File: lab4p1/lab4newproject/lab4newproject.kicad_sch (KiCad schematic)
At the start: 10 parts, among them J1 9V, U1 NE555D

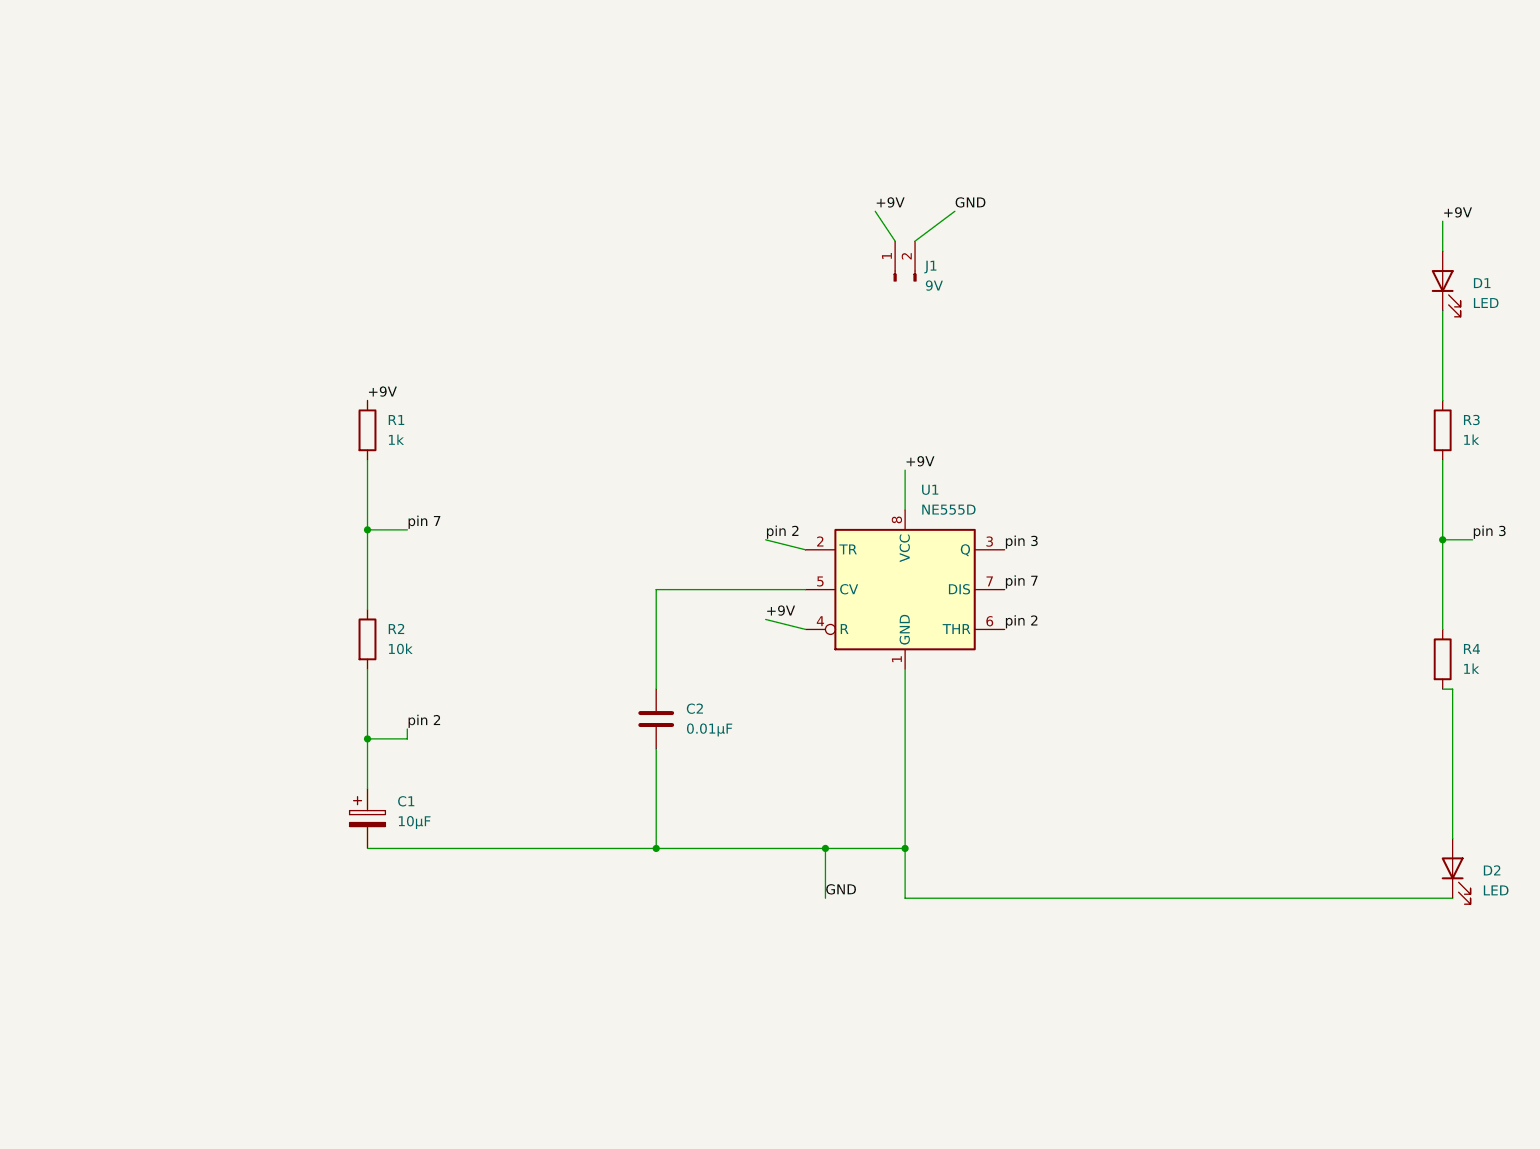
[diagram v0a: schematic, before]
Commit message: PCB design pics
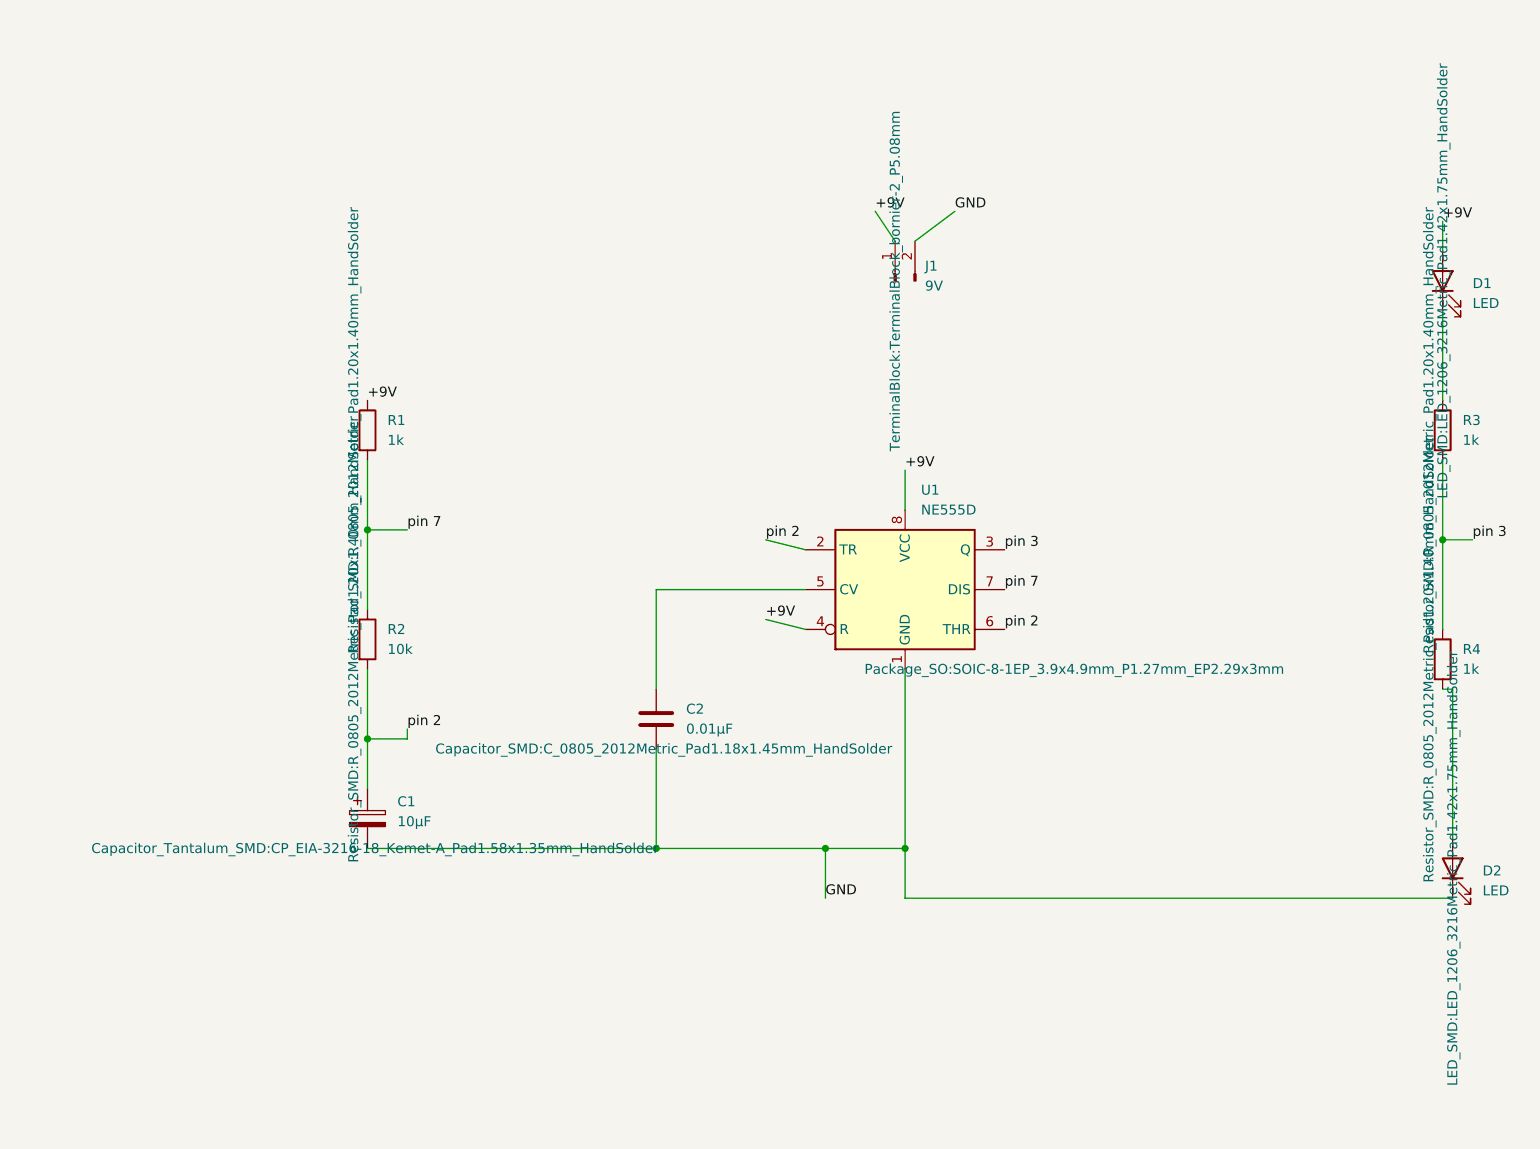
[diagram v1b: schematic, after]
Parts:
- C1: footprint (none) -> Capacitor_Tantalum_SMD:CP_EIA-3216-18_Kemet-A_Pad1.58x1.35mm_HandSolder
- C2: footprint (none) -> Capacitor_SMD:C_0805_2012Metric_Pad1.18x1.45mm_HandSolder
- D1, D2: footprint (none) -> LED_SMD:LED_1206_3216Metric_Pad1.42x1.75mm_HandSolder
- J1: footprint (none) -> TerminalBlock:TerminalBlock_bornier-2_P5.08mm
- R1, R2, R3, R4: footprint (none) -> Resistor_SMD:R_0805_2012Metric_Pad1.20x1.40mm_HandSolder
- U1: footprint Package_SO:SOIC-8_3.9x4.9mm_P1.27mm -> Package_SO:SOIC-8-1EP_3.9x4.9mm_P1.27mm_EP2.29x3mm
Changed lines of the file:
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@@
       (effects (font (size 1.27 1.27)) (justify right))
     )
-    (property "Footprint" "" (id 2) (at 207.01 34.29 0)
-      (effects (font (size 1.27 1.27)) hide)
-    )
+    (property "Footprint" "LED_SMD:LED_1206_3216Metric_Pad1.42x1.75mm_HandSolder" (id 2) (at 207.01 34.29 0))
     (property "Datasheet" "~" (id 3) (at 207.01 34.29 0)
       (effects (font (size 1.27 1.27)) hide)
@@
       (effects (font (size 1.27 1.27)) (justify right))
     )
-    (property "Footprint" "" (id 2) (at 137.16 34.29 0)
-      (effects (font (size 1.27 1.27)) hide)
-    )
+    (property "Footprint" "TerminalBlock:TerminalBlock_bornier-2_P5.08mm" (id 2) (at 137.16 34.29 0))
     (property "Datasheet" "~" (id 3) (at 137.16 34.29 0)
       (effects (font (size 1.27 1.27)) hide)
@@
       (effects (font (size 1.27 1.27)) (justify right))
     )
-    (property "Footprint" "" (id 2) (at 208.28 109.22 0)
-      (effects (font (size 1.27 1.27)) hide)
-    )
+    (property "Footprint" "LED_SMD:LED_1206_3216Metric_Pad1.42x1.75mm_HandSolder" (id 2) (at 208.28 109.22 0))
     (property "Datasheet" "~" (id 3) (at 208.28 109.22 0)
       (effects (font (size 1.27 1.27)) hide)
@@
       (effects (font (size 1.27 1.27)) (justify left))
     )
-    (property "Footprint" "" (id 2) (at 205.232 82.55 90)
-      (effects (font (size 1.27 1.27)) hide)
-    )
+    (property "Footprint" "Resistor_SMD:R_0805_2012Metric_Pad1.20x1.40mm_HandSolder" (id 2) (at 205.232 82.55 90))
     (property "Datasheet" "~" (id 3) (at 207.01 82.55 0)
       (effects (font (size 1.27 1.27)) hide)
@@
       (effects (font (size 1.27 1.27)) (justify left))
     )
-    (property "Footprint" "" (id 2) (at 70.8152 106.68 0)
-      (effects (font (size 1.27 1.27)) hide)
-    )
+    (property "Footprint" "Capacitor_Tantalum_SMD:CP_EIA-3216-18_Kemet-A_Pad1.58x1.35mm_HandSolder" (id 2) (at 70.8152 106.68 0))
     (property "Datasheet" "~" (id 3) (at 69.85 102.87 0)
       (effects (font (size 1.27 1.27)) hide)
@@
       (effects (font (size 1.27 1.27)) (justify left))
     )
-    (property "Footprint" "" (id 2) (at 68.072 53.34 90)
-      (effects (font (size 1.27 1.27)) hide)
-    )
+    (property "Footprint" "Resistor_SMD:R_0805_2012Metric_Pad1.20x1.40mm_HandSolder" (id 2) (at 68.072 53.34 90))
     (property "Datasheet" "~" (id 3) (at 69.85 53.34 0)
       (effects (font (size 1.27 1.27)) hide)
@@
       (effects (font (size 1.27 1.27)) (justify left))
     )
-    (property "Footprint" "Package_SO:SOIC-8_3.9x4.9mm_P1.27mm" (id 2) (at 160.02 83.82 0)
-      (effects (font (size 1.27 1.27)) hide)
-    )
+    (property "Footprint" "Package_SO:SOIC-8-1EP_3.9x4.9mm_P1.27mm_EP2.29x3mm" (id 2) (at 160.02 83.82 0))
     (property "Datasheet" "http://www.ti.com/lit/ds/symlink/ne555.pdf" (id 3) (at 160.02 83.82 0)
       (effects (font (size 1.27 1.27)) hide)
@@
       (effects (font (size 1.27 1.27)) (justify left))
     )
-    (property "Footprint" "" (id 2) (at 107.6452 93.98 0)
-      (effects (font (size 1.27 1.27)) hide)
-    )
+    (property "Footprint" "Capacitor_SMD:C_0805_2012Metric_Pad1.18x1.45mm_HandSolder" (id 2) (at 107.6452 93.98 0))
     (property "Datasheet" "~" (id 3) (at 106.68 90.17 0)
       (effects (font (size 1.27 1.27)) hide)
@@
       (effects (font (size 1.27 1.27)) (justify left))
     )
-    (property "Footprint" "" (id 2) (at 68.072 80.01 90)
-      (effects (font (size 1.27 1.27)) hide)
-    )
+    (property "Footprint" "Resistor_SMD:R_0805_2012Metric_Pad1.20x1.40mm_HandSolder" (id 2) (at 68.072 80.01 90))
     (property "Datasheet" "~" (id 3) (at 69.85 80.01 0)
       (effects (font (size 1.27 1.27)) hide)
@@
       (effects (font (size 1.27 1.27)) (justify left))
     )
-    (property "Footprint" "" (id 2) (at 205.232 53.34 90)
-      (effects (font (size 1.27 1.27)) hide)
-    )
+    (property "Footprint" "Resistor_SMD:R_0805_2012Metric_Pad1.20x1.40mm_HandSolder" (id 2) (at 205.232 53.34 90))
     (property "Datasheet" "~" (id 3) (at 207.01 53.34 0)
       (effects (font (size 1.27 1.27)) hide)
@@
   (symbol_instances
     (path "/9c9f3f99-31c3-40cb-848d-7689503b5f84"
-      (reference "C1") (unit 1) (value "10μF") (footprint "")
+      (reference "C1") (unit 1) (value "10μF") (footprint "Capacitor_Tantalum_SMD:CP_EIA-3216-18_Kemet-A_Pad1.58x1.35mm_HandSolder")
     )
     (path "/d43c6e1d-e6d1-4d04-a32f-7f9141b5e258"
-      (reference "C2") (unit 1) (value "0.01μF") (footprint "")
+      (reference "C2") (unit 1) (value "0.01μF") (footprint "Capacitor_SMD:C_0805_2012Metric_Pad1.18x1.45mm_HandSolder")
     )
     (path "/00681a6e-2c14-445a-b819-0193c48afd5d"
-      (reference "D1") (unit 1) (value "LED") (footprint "")
+      (reference "D1") (unit 1) (value "LED") (footprint "LED_SMD:LED_1206_3216Metric_Pad1.42x1.75mm_HandSolder")
     )
     (path "/3306eaa7-cedb-4c25-a1b1-b3b4827d0b4a"
-      (reference "D2") (unit 1) (value "LED") (footprint "")
+      (reference "D2") (unit 1) (value "LED") (footprint "LED_SMD:LED_1206_3216Metric_Pad1.42x1.75mm_HandSolder")
     )
     (path "/0a9f1a3d-d8a9-488b-bd68-c02a8d0d1021"
-      (reference "J1") (unit 1) (value "9V") (footprint "")
+      (reference "J1") (unit 1) (value "9V") (footprint "TerminalBlock:TerminalBlock_bornier-2_P5.08mm")
     )
     (path "/b256dc72-2f5e-47b4-841d-fecd9d40720d"
-      (reference "R1") (unit 1) (value "1k") (footprint "")
+      (reference "R1") (unit 1) (value "1k") (footprint "Resistor_SMD:R_0805_2012Metric_Pad1.20x1.40mm_HandSolder")
     )
     (path "/d663f8eb-1448-4cfd-9129-a5d32d31c4b3"
-      (reference "R2") (unit 1) (value "10k") (footprint "")
+      (reference "R2") (unit 1) (value "10k") (footprint "Resistor_SMD:R_0805_2012Metric_Pad1.20x1.40mm_HandSolder")
     )
     (path "/eab8c07f-d5aa-4ccb-b85c-0d1e7d9beb0b"
-      (reference "R3") (unit 1) (value "1k") (footprint "")
+      (reference "R3") (unit 1) (value "1k") (footprint "Resistor_SMD:R_0805_2012Metric_Pad1.20x1.40mm_HandSolder")
     )
     (path "/63bc51c2-a3cc-417e-b378-c0668083d6c9"
-      (reference "R4") (unit 1) (value "1k") (footprint "")
+      (reference "R4") (unit 1) (value "1k") (footprint "Resistor_SMD:R_0805_2012Metric_Pad1.20x1.40mm_HandSolder")
     )
     (path "/bd855e8d-a5aa-44b1-9706-ba50d042cbbf"
-      (reference "U1") (unit 1) (value "NE555D") (footprint "Package_SO:SOIC-8_3.9x4.9mm_P1.27mm")
+      (reference "U1") (unit 1) (value "NE555D") (footprint "Package_SO:SOIC-8-1EP_3.9x4.9mm_P1.27mm_EP2.29x3mm")
     )
   )
